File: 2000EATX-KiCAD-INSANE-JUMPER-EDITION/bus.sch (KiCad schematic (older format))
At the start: 26 parts, among them U302 74HCT32, U800 BUSTER, U801 RTC62423, U802 74HCT138, U803 74HCT08, U804 74LS148

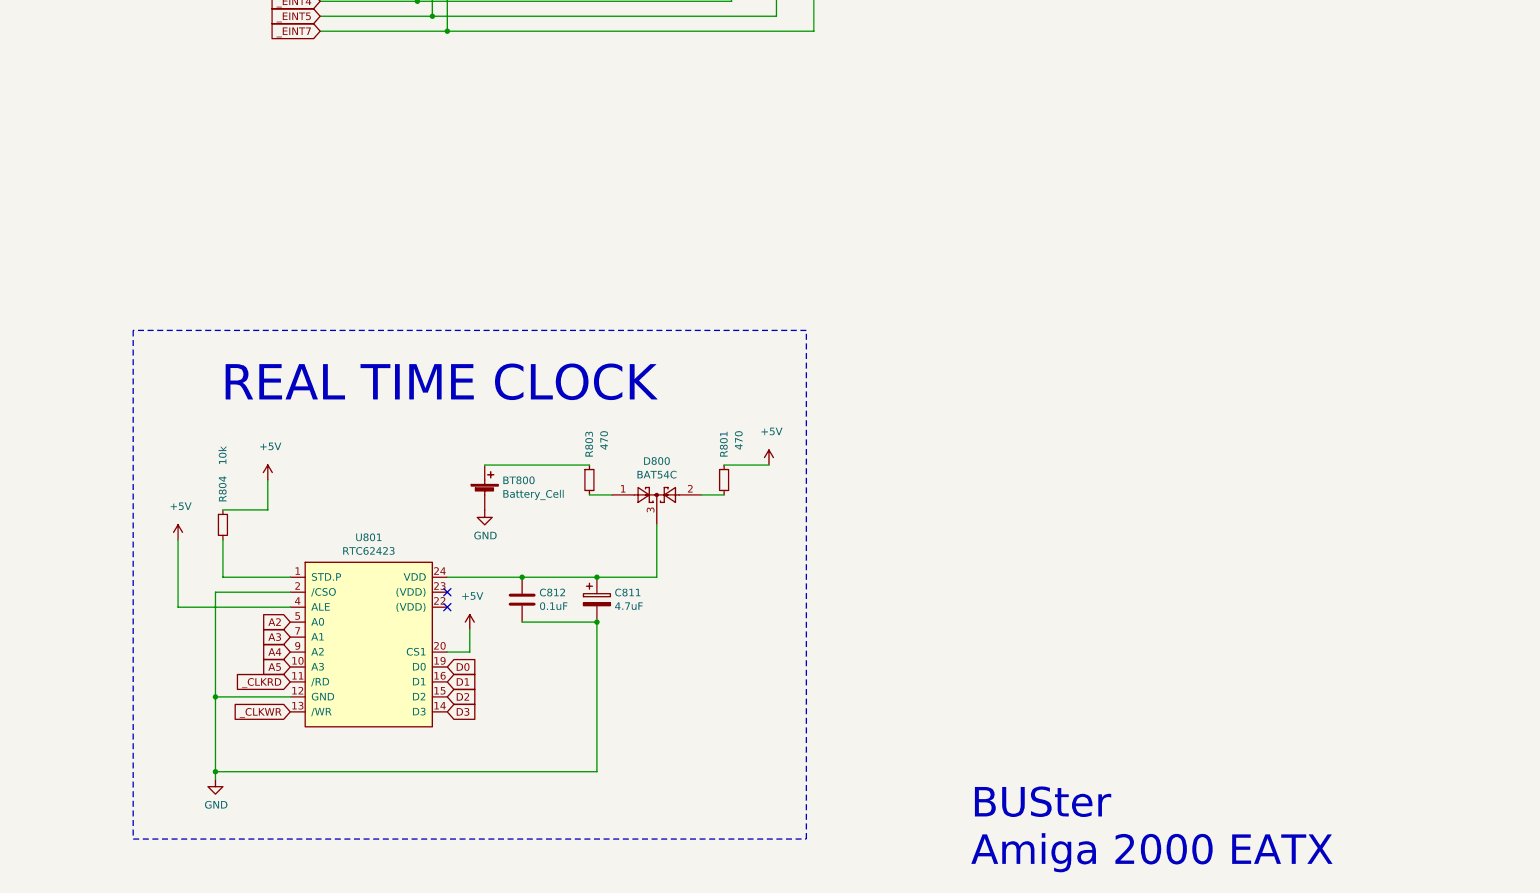
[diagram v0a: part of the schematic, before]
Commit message: Add files via upload
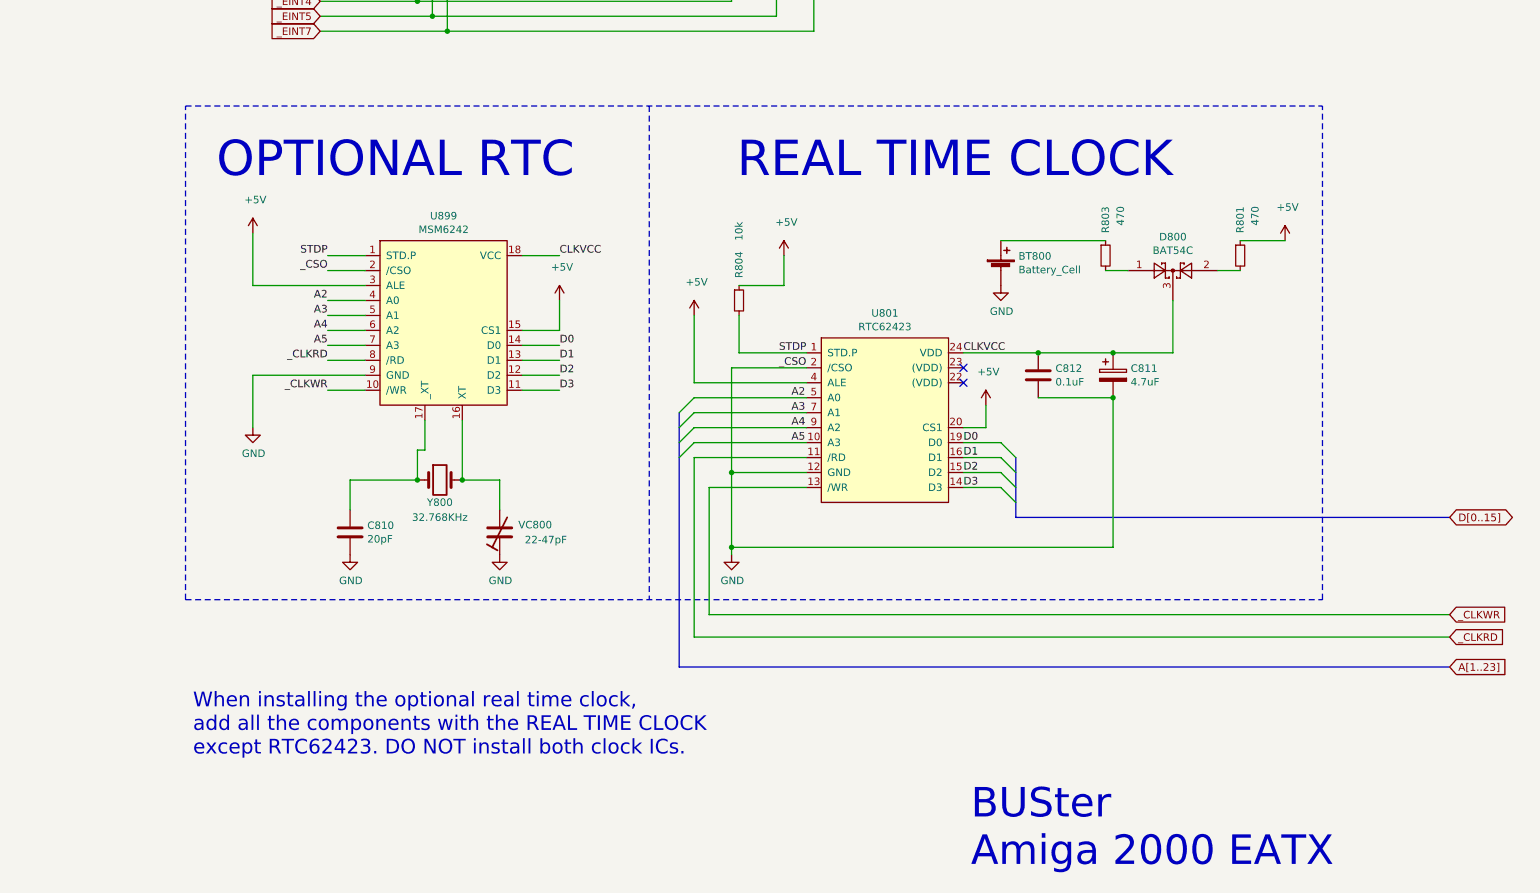
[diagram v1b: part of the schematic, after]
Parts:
- added C810: 20pF, Capacitor_SMD:C_1206_3216Metric, symbol Device:C
- added U899: MSM6242, Package_DIP:DIP-18_W7.62mm_Socket, symbol Amiga-Library:MSM6242
- added VC800: 22-47pF, AmigaFootprints:TrimmerCap, symbol Device:CTRIM
- added Y800: 32.768KHz, Crystal:Crystal_SMD_3215-2Pin_3.2x1.5mm, symbol Device:Crystal
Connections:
- net +5V: now also U899.15 (CS1), U899.3 (ALE)
- net A2: now also U899.4 (A0)
- net A3: now also U899.5 (A1)
- net A4: now also U899.6 (A2)
- net A5: now also U899.7 (A3)
- net D0: now also U899.14 (D0)
- net D1: now also U899.13 (D1)
- net D2: now also U899.12 (D2)
- net D3: now also U899.11 (D3)
- net GND: now also C810.2, U899.2 (/CSO), U899.9 (GND), VC800.1
- net _CLKRD: now also U899.8 (/RD)
- net _CLKWR: now also U899.10 (/WR)
- net STDP: now reaches R804.2, U801.1 (STD.P)
- net STDP: now also U899.1 (STD.P)
- net CLKVCC: now reaches C811.1, C812.1, D800.3, U801.24 (VDD)
- net CLKVCC: now also U899.18 (VCC)
- new net: U899.16 (XT), VC800.2, Y800.2
- new net: C810.1, U899.17 (_XT), Y800.1
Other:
- note added: "OPTIONAL RTC"
- note added: "When installing the optional real time clock,\nadd all the components with the REAL TIME CLOCK\nexcept RTC62423. DO NOT install both clock ICs."
- moved on the sheet: BT800, C811, C812, D800, R801, R803, R804, U801

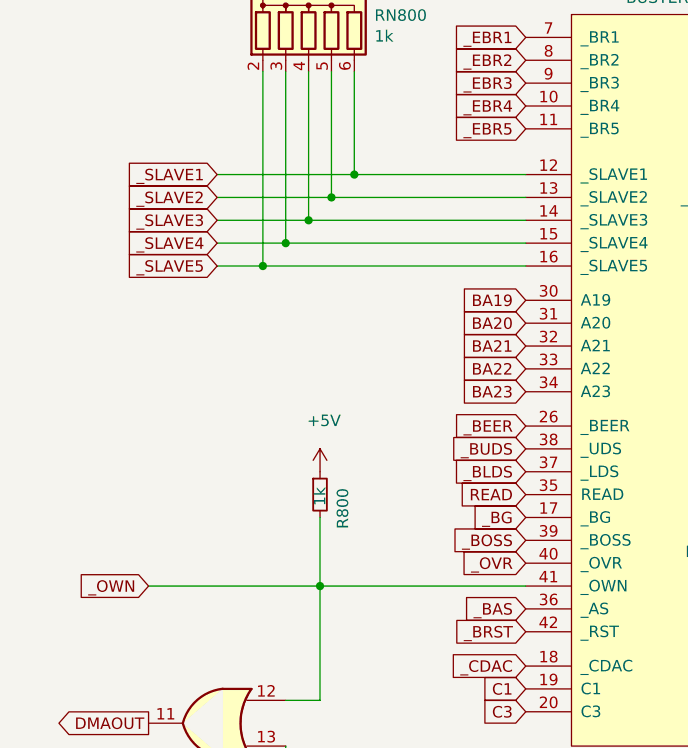
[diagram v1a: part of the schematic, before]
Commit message: Add files via upload
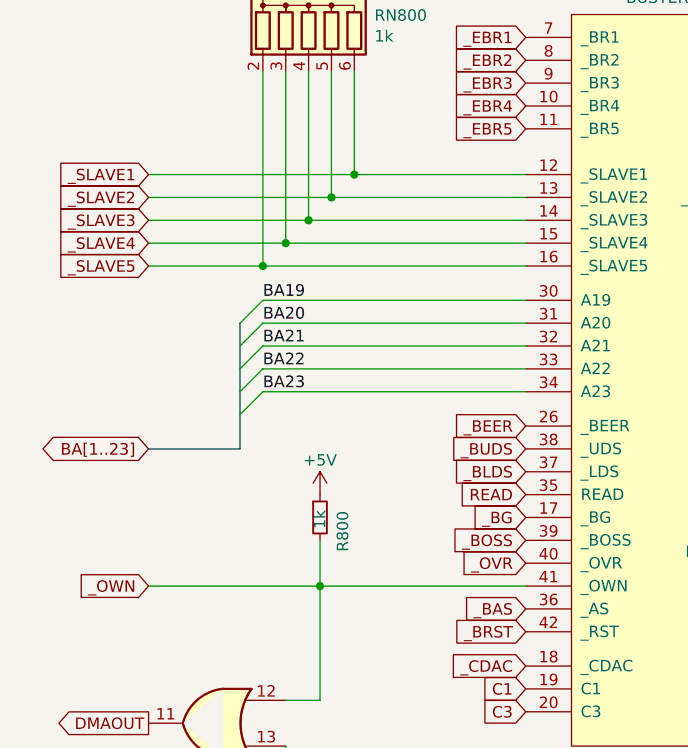
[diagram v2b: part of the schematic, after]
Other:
- moved on the sheet: R800
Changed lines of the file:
@@
 Connection ~ 1500 3550
 Wire Wire Line
-	1500 3550 1300 3550
+	1500 3550 1000 3550
 Wire Wire Line
 	1600 2700 1600 3450
 Connection ~ 1600 3450
 Wire Wire Line
-	1600 3450 1300 3450
+	1600 3450 1000 3450
 Wire Wire Line
 	1700 2700 1700 3350
 Connection ~ 1700 3350
 Wire Wire Line
-	1700 3350 1300 3350
+	1700 3350 1000 3350
 Wire Wire Line
 	1800 2700 1800 3250
 Connection ~ 1800 3250
 Wire Wire Line
-	1800 3250 1300 3250
+	1800 3250 1000 3250
 Wire Wire Line
 	1900 2700 1900 3150
 Connection ~ 1900 3150
 Wire Wire Line
-	1900 3150 1300 3150
-Text GLabel 1300 3150 0    50   Input ~ 0
+	1900 3150 1000 3150
+Text GLabel 1000 3150 0    50   Input ~ 0
 _SLAVE1
-Text GLabel 1300 3250 0    50   Input ~ 0
+Text GLabel 1000 3250 0    50   Input ~ 0
 _SLAVE2
-Text GLabel 1300 3350 0    50   Input ~ 0
+Text GLabel 1000 3350 0    50   Input ~ 0
 _SLAVE3
-Text GLabel 1300 3450 0    50   Input ~ 0
+Text GLabel 1000 3450 0    50   Input ~ 0
 _SLAVE4
-Text GLabel 1300 3550 0    50   Input ~ 0
+Text GLabel 1000 3550 0    50   Input ~ 0
 _SLAVE5
-Text GLabel 2650 3700 0    50   Input ~ 0
-BA19
-Text GLabel 2650 3800 0    50   Input ~ 0
-BA20
-Text GLabel 2650 3900 0    50   Input ~ 0
-BA21
-Text GLabel 2650 4100 0    50   Input ~ 0
-BA23
-Text GLabel 2650 4000 0    50   Input ~ 0
-BA22
 Text GLabel 2650 4250 0    50   Input ~ 0
 _BEER
@@
 L Device:R_Small R800
 U 1 1 605ACB88
-P 1750 4550
-F 0 "R800" V 1850 4400 50  0000 L CNN
-F 1 "1k" V 1750 4500 50  0000 L CNN
-F 2 "Resistor_SMD:R_1206_3216Metric" H 1750 4550 50  0001 C CNN
-F 3 "~" H 1750 4550 50  0001 C CNN
-	1    1750 4550
+P 1750 4650
+F 0 "R800" V 1850 4500 50  0000 L CNN
+F 1 "1k" V 1750 4600 50  0000 L CNN
+F 2 "Resistor_SMD:R_1206_3216Metric" H 1750 4650 50  0001 C CNN
+F 3 "~" H 1750 4650 50  0001 C CNN
+	1    1750 4650
 	1    0    0    -1
 $EndComp
@@
 L power:+5V #PWR0226
 U 1 1 605B0A1C
-P 1750 4450
-F 0 "#PWR0226" H 1750 4300 50  0001 C CNN
-F 1 "+5V" H 1767 4673 50  0000 C CNN
-F 2 "" H 1750 4450 50  0001 C CNN
-F 3 "" H 1750 4450 50  0001 C CNN
-	1    1750 4450
+P 1750 4550
+F 0 "#PWR0226" H 1750 4400 50  0001 C CNN
+F 1 "+5V" H 1750 4700 50  0000 C CNN
+F 2 "" H 1750 4550 50  0001 C CNN
+F 3 "" H 1750 4550 50  0001 C CNN
+	1    1750 4550
 	1    0    0    -1
 $EndComp
@@
 	1000 4950 1750 4950
 Wire Wire Line
-	1750 4650 1750 4950
+	1750 4750 1750 4950
 Connection ~ 1750 4950
 Wire Wire Line
@@
 Text Notes 7150 9100 0    98   ~ 0
 When installing the optional real time clock,\nadd all the components with the REAL TIME CLOCK\nexcept RTC62423. DO NOT install both clock ICs.
+Wire Wire Line
+	2650 4100 1500 4100
+Entry Wire Line
+	1500 4100 1400 4200
+Wire Wire Line
+	2650 4000 1500 4000
+Wire Wire Line
+	2650 3900 1500 3900
+Wire Wire Line
+	2650 3800 1500 3800
+Wire Wire Line
+	2650 3700 1500 3700
+Entry Wire Line
+	1500 4000 1400 4100
+Entry Wire Line
+	1500 3900 1400 4000
+Entry Wire Line
+	1500 3800 1400 3900
+Entry Wire Line
+	1500 3700 1400 3800
+Wire Bus Line
+	1400 4350 1000 4350
+Text Label 1500 4100 0    51   ~ 0
+BA23
+Text Label 1500 4000 0    51   ~ 0
+BA22
+Text Label 1500 3900 0    51   ~ 0
+BA21
+Text Label 1500 3800 0    51   ~ 0
+BA20
+Text Label 1500 3700 0    51   ~ 0
+BA19
+Text GLabel 1000 4350 0    51   BiDi ~ 0
+BA[1..23]
 Wire Bus Line
 	10400 6800 10400 8500
 Wire Bus Line
 	12650 7100 12650 7500
+Wire Bus Line
+	1400 3800 1400 4350
 $EndSCHEMATC
